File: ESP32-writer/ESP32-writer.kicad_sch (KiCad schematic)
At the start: 27 parts, among them J1 USB2.0_C, J2 USB2.0_C, J3 ESP-Prog-ProgramCOM-SEND, J4 UART-OUTPUT, Q1 2N7002, Q2 2N7002, U1 AMS1117-3.3, U2 CH340G, Y1 12M

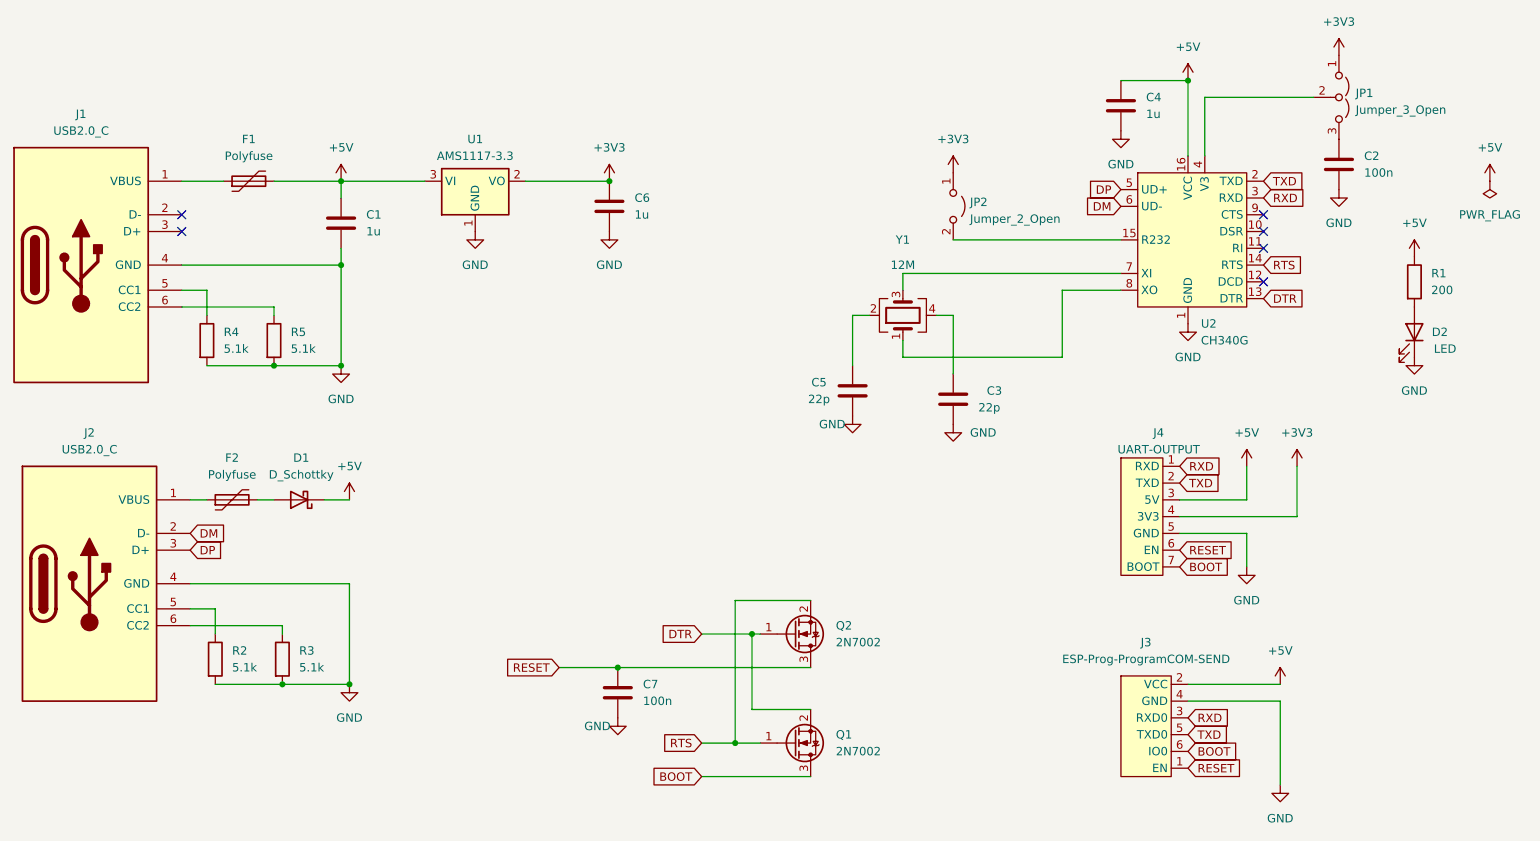
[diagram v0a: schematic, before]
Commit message: type ch340g
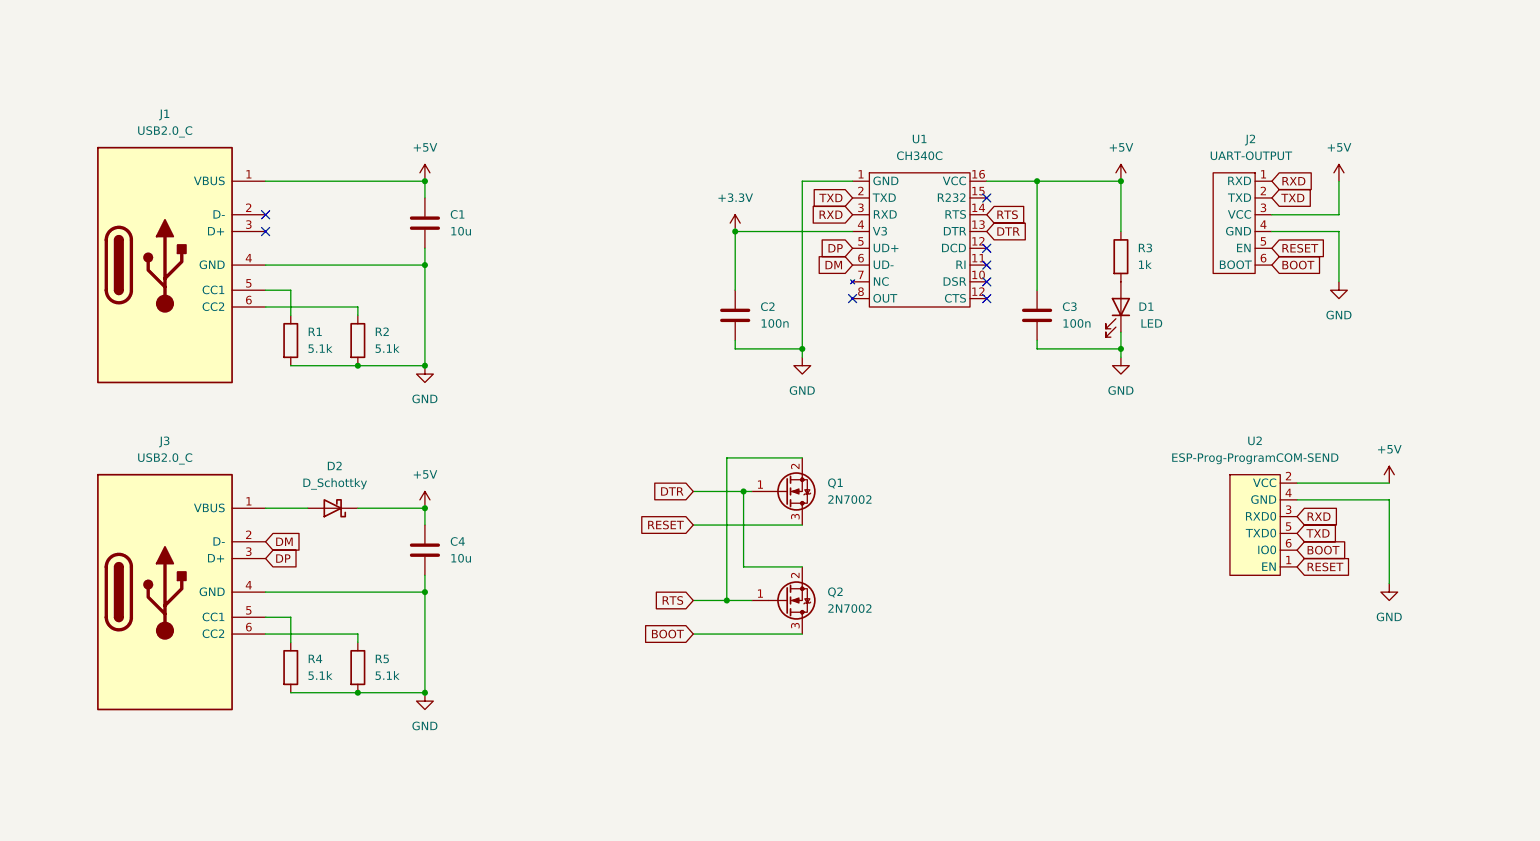
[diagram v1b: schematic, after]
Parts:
- removed C3, C5: 22p, $74th:Capacitor_0805_2012, symbol Device:C
- removed C6: 1u, $74th:Capacitor_0805_2012, symbol Device:C
- removed C7: 100n, $74th:Capacitor_0805_2012, symbol Device:C
- removed F1, F2: Polyfuse, $74th:ResettableFuse_KT6-1100SMDI, symbol Device:Polyfuse
- removed JP1: Jumper_3_Open, Jumper:SolderJumper-3_P1.3mm_Open_RoundedPad1.0x1.5mm_NumberLabels, symbol Jumper:Jumper_3_Open
- removed JP2: Jumper_2_Open, Jumper:SolderJumper-2_P1.3mm_Open_RoundedPad1.0x1.5mm, symbol Jumper:Jumper_2_Open
- removed U1: AMS1117-3.3, Package_TO_SOT_SMD:SOT-223-3_TabPin2, symbol Regulator_Linear:AMS1117-3.3
- removed Y1: 12M, $74th:Crystal_SMD_3225-4Pin_3.2x2.5mm_HandSoldering, symbol Device:Crystal_GND24
- added C4: 10u, $74th:Capacitor_0805_2012, symbol Device:C
- C1: value 1u -> 10u
- C3: renamed from C4; value 1u -> 100n
- J1: footprint $74th:USB-C-12-Pin-MidMount-ali-v5 -> $74th:USB-C-12-Pin-MidMount-ali-v4
- J2: renamed from J4; symbol esp32-dev-board:UART-OUTPUT-v2 -> esp32-dev-board:UART-OUTPUT
- J3: renamed from J2; footprint $74th:USB-C-12-Pin-MidMount-ali-v5 -> $74th:USB-C-12-Pin-MidMount-ali-v4
- R3: renamed from R1; value 200 -> 1k
- U1: renamed from U2; value CH340G -> CH340C; symbol $74th:CH340G -> esp32-dev-board:CH340C
- renumbered D2 to D1, D1 to D2, Q2 to Q1, Q1 to Q2, R4 to R1, R5 to R2, R2 to R4, R3 to R5, J3 to U2
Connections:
- net +3V3 is gone; now on net GND: J2.4 (GND)
- net +5V: now also J1.1 (VBUS), C4.1
- net BOOT: now also J2.6 (BOOT); no longer J2.7 (BOOT)
- net GND: now also C4.2; no longer J2.5 (GND)
- net RESET: now also J2.5 (EN); no longer J2.6 (EN)
- net at D2.2 (A): now also J3.1 (VBUS)
- net +3.3V: now reaches U1.4 (V3)
- net +3.3V: now also C2.1
- no-connect marks 6 -> 8
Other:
- moved on the sheet: C1, C2, C3, D1, D2, J1, J3, Q1, Q2, R1, R2, R3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
